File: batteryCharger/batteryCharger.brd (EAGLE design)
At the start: 44.1 x 67 mm, 73 parts, among them J1 B4P-VH(LF)(SN), Q1 SIR414DP-T1-GE3, Q2 SI7635DP-T1-GE3, Q3 SI7635DP-T1-GE3, Q4 SIR414DP-T1-GE3, Q5 SI7635DP-T1-GE3

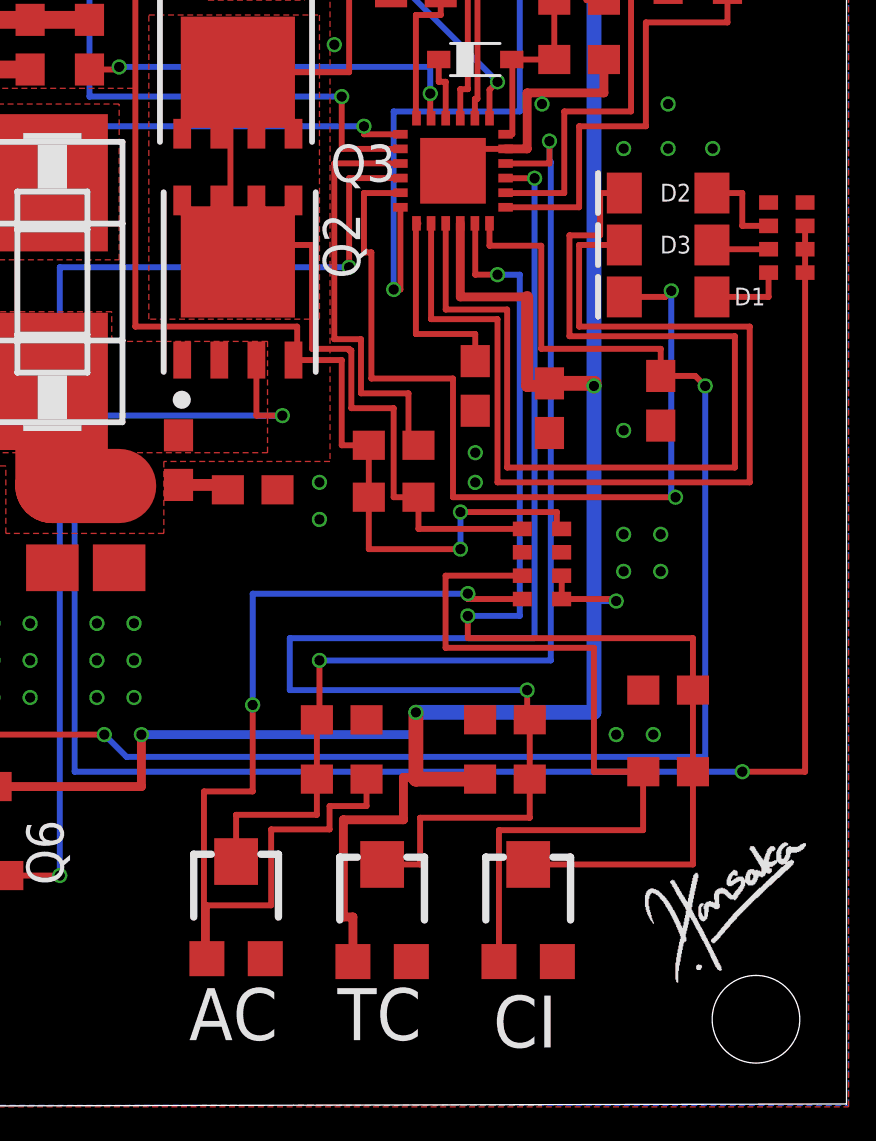
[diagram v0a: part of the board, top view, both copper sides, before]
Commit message: final board file
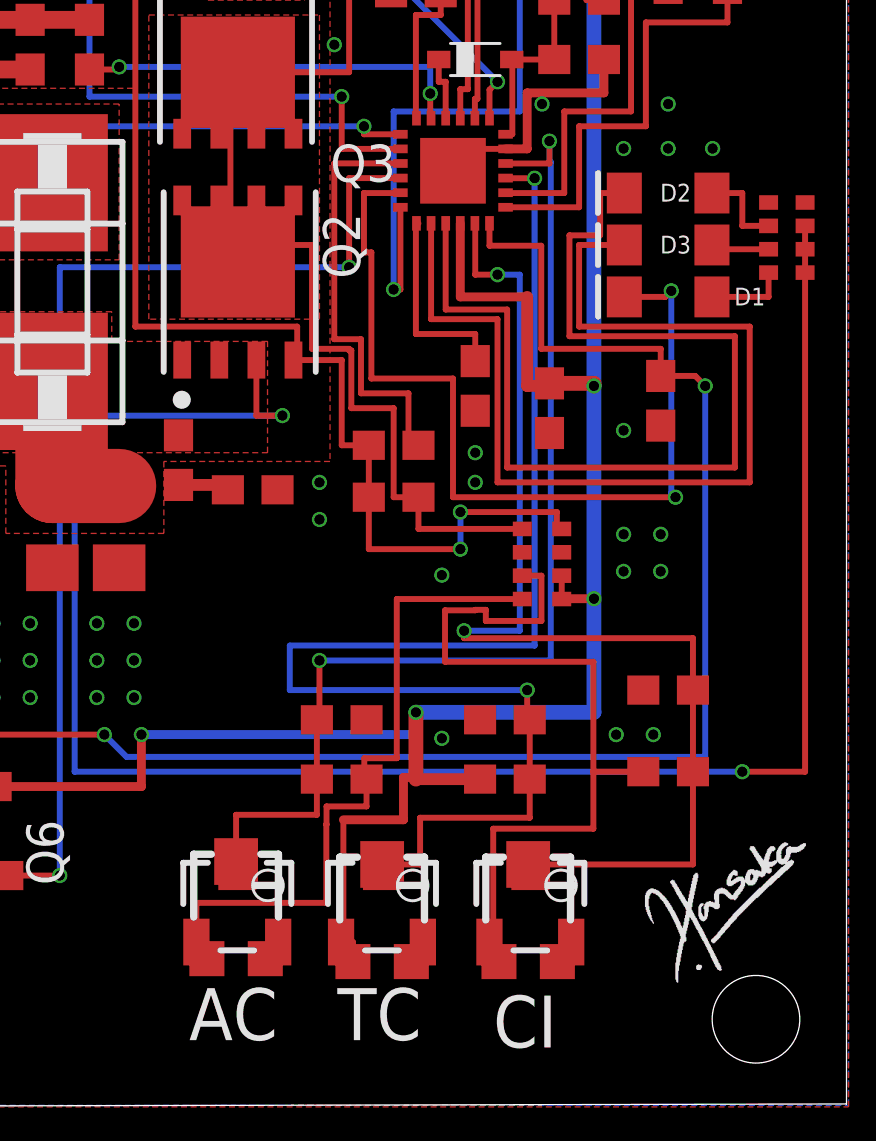
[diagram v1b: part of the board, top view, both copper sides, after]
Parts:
- added R21, R22, R23: (no value), pot:3223W
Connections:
- removed net N$11: R5.1, RN2.7, TM1.1
- removed net N$9: R19.1, RN2.8, TM3.1
- new net ACSET_TRIM: R19.1, R23.1, RN2.8, TM3.1
- new net ISET1_TRIM: R21.1, R5.1, RN2.7, TM1.1
- net ACSET: now also R23.2
- net GND: now also R21.3, R22.3, R23.3
- net ISET1: now also R21.2
- net ISET2: now also R22.2
- net VREF: now also R22.1
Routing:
- net N$9: track 35.3 -> 0.00 mm, vias 2 -> 0
- net ISET1_TRIM: track 0.00 -> 29.2 mm
- net N$11: track 27.5 -> 0.00 mm
- net ACSET_TRIM: track 0.00 -> 24.1 mm
- net GND: track 11.7 -> 13.1 mm, vias 120 -> 122
- net ISET1: track 38.6 -> 39.2 mm
- net VREF: track 111.8 -> 111.3 mm
